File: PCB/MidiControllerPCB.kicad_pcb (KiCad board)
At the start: 2 copper layers, 202.8 x 137.6 mm, 62 parts, among them J1 OLED_Display, J2 fan_header, J24 TRS_Midi_1, J25 TRS_Midi_2, J3 TRS_Midi_3, J35 Raspberry_Pi_2_3, J4 TRS_Midi_4, J41 PIC_debug, J7 DIN_5, J8 DIN_5, SW1 SW_SPST, SW2 SW_SPST, SW3 SW_SPST, SW4 SW_SPST, SW5 SW_SPST, SW6 RGB_Rotary_Enc_PB, U10 PIC18F26K80_IML, U2 MCP23017_ML, U5 CD4050BCN

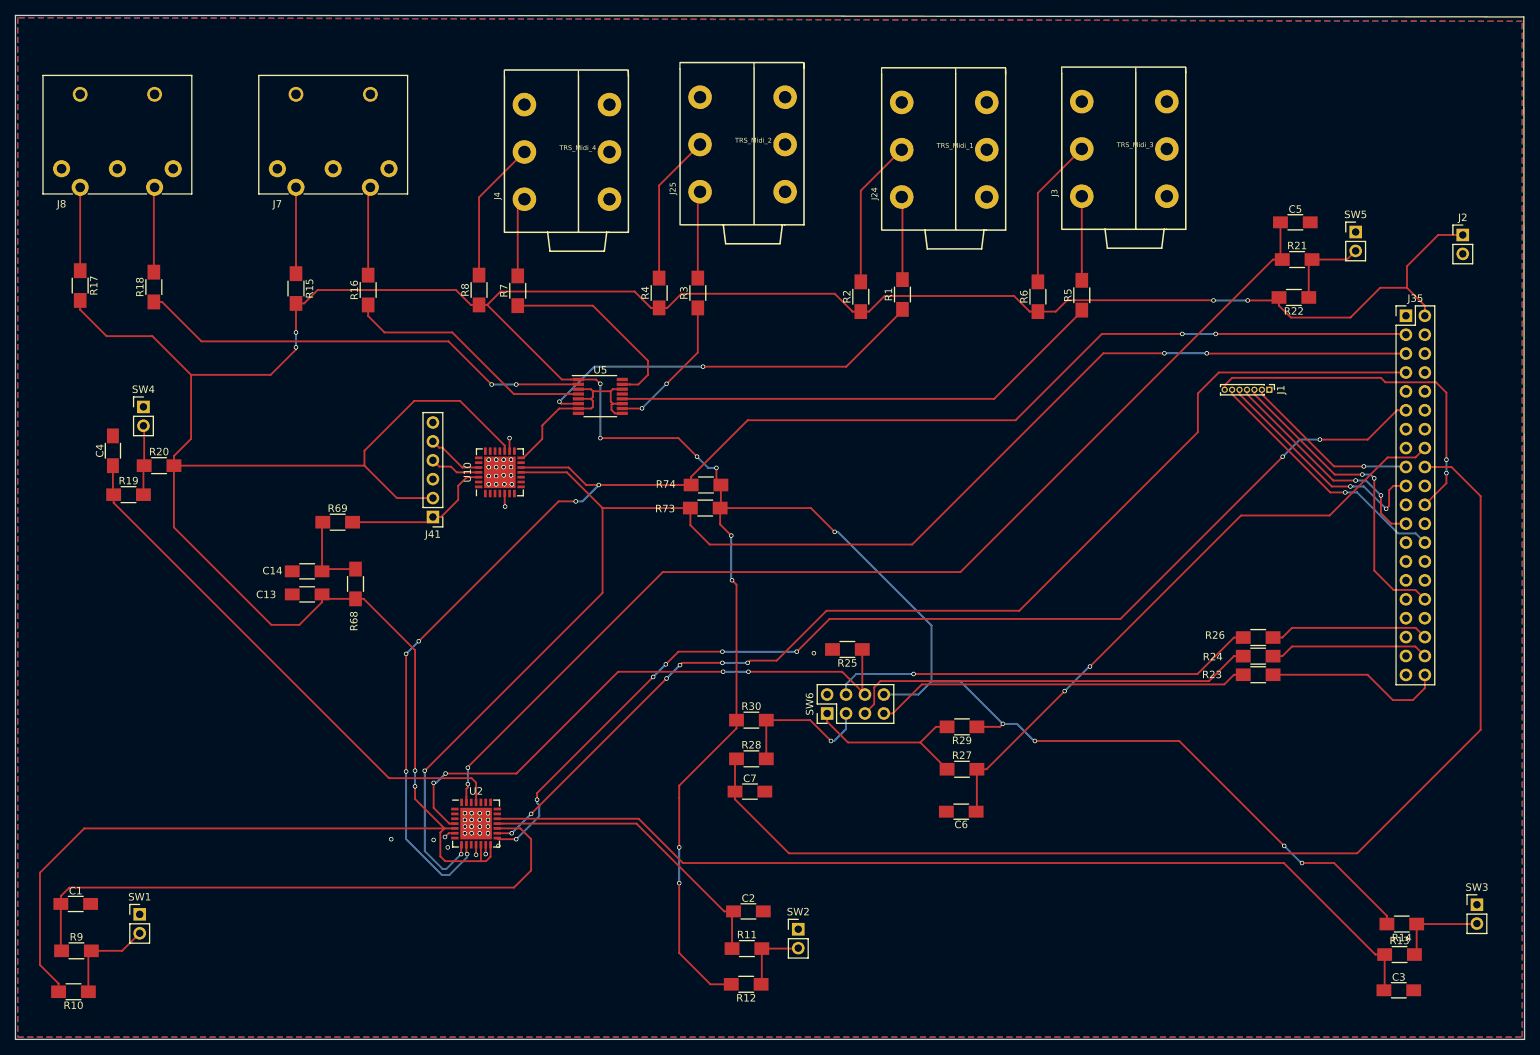
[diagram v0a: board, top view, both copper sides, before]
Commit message: modify pcb
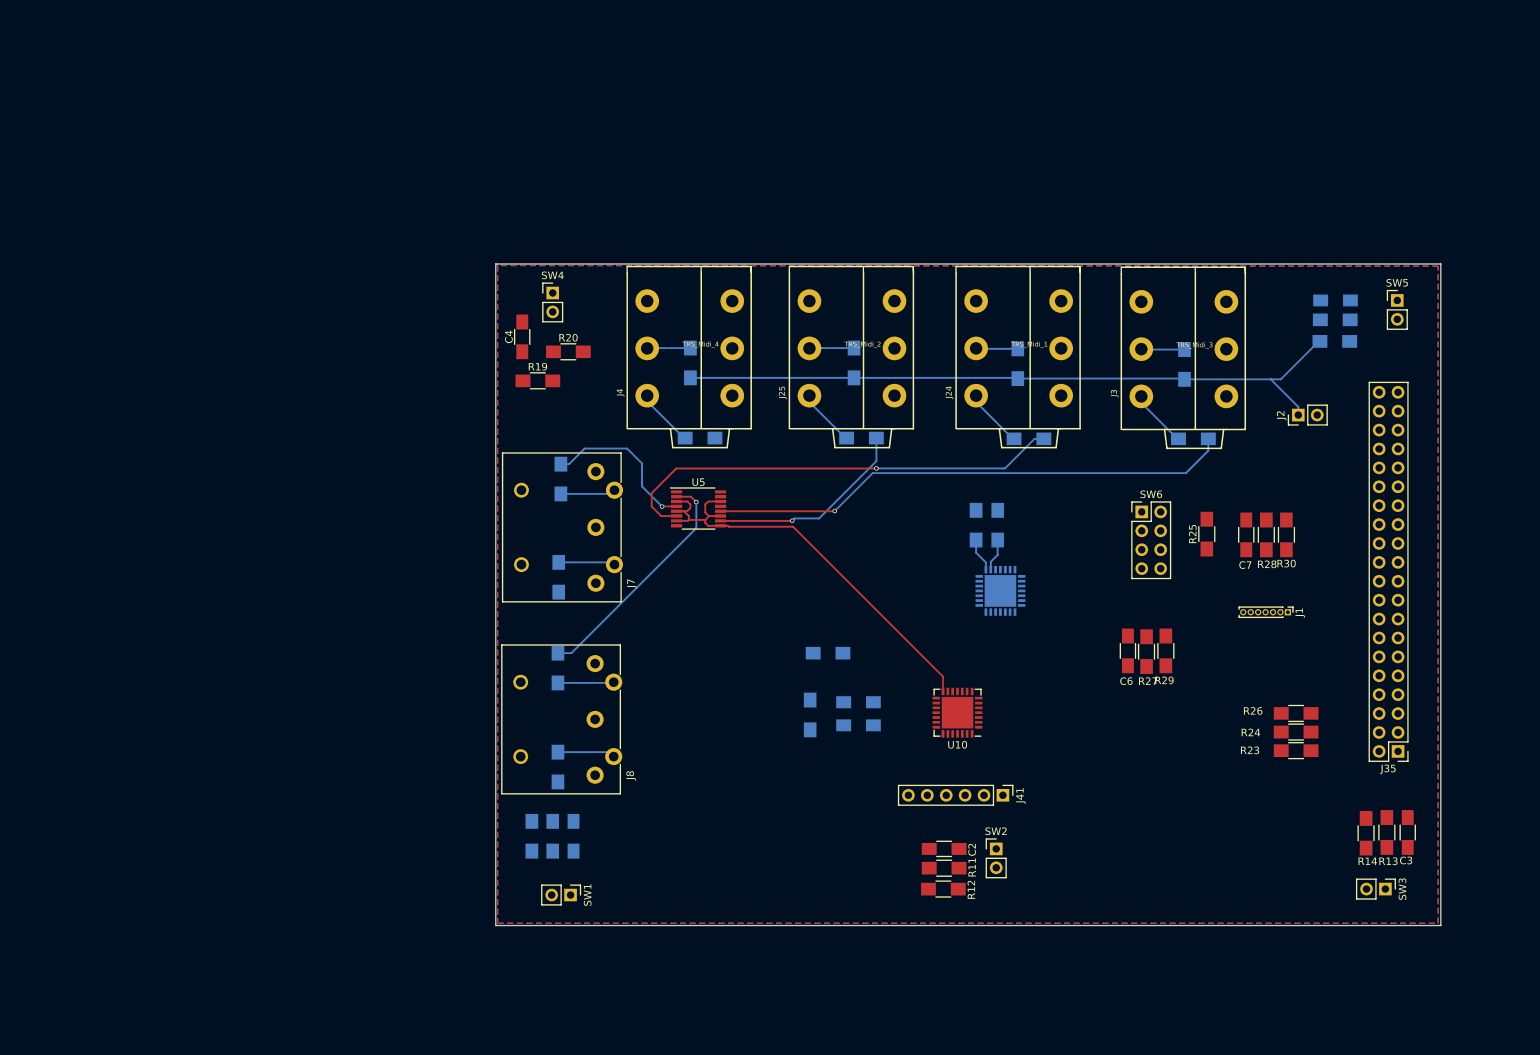
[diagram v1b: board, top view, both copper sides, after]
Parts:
- C1, C13, C14, C5, R1, R10, R15, R16, R17, R18, R2, R21, R22, R3, R4, R5, R6, R68, R69, R7, R73, R74, R8, R9, U2: moved to B.Cu
- moved J8 108.6 mm to (109.7, 123.9), turned to 90 degrees
- moved R17 91.1 mm to (104.7, 122.8)
- moved J41 85.2 mm to (164.5, 126.6), turned to 270 degrees
- moved U2 77.1 mm to (164.2, 99.1)
- moved C13 76.2 mm to (145.1, 117.2), turned to 180 degrees
- moved C14 76.2 mm to (145.1, 114.1), turned to 180 degrees
- moved R30 76.1 mm to (202.6, 91.6), turned to 270 degrees
- moved R28 75.5 mm to (199.9, 91.6), turned to 270 degrees
- moved C7 75.1 mm to (197.2, 91.6), turned to 270 degrees
- moved R18 74.6 mm to (104.7, 109.5), turned to 270 degrees
- moved J7 70.2 mm to (109.8, 98.1), turned to 90 degrees
- moved U10 69.5 mm to (158.4, 115.5), turned to 180 degrees
- moved R69 68.2 mm to (141.0, 107.5), turned to 180 degrees
- moved C1 67.5 mm to (106.8, 132.1), turned to 270 degrees
- moved R9 65.8 mm to (104.0, 132.1), turned to 270 degrees
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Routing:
- net VCC: track 713.8 -> 93.1 mm, vias 19 -> 0
- net Net-(J35-Pad3): track 202.1 -> 4.37 mm, vias 8 -> 0
- net Net-(J35-Pad5): track 198.9 -> 4.53 mm, vias 4 -> 0
- net RotEncB: track 156.1 -> 0.00 mm
- net Net-(J35-Pad7): track 150.8 -> 0.00 mm, vias 6 -> 0
- net Net-(J35-Pad11): track 148.3 -> 0.00 mm, vias 8 -> 0
- net FootSw5: track 147.6 -> 0.00 mm, vias 2 -> 0
- net FootSw3: track 131.7 -> 0.00 mm
- net RotEncA: track 83.8 -> 0.00 mm, vias 2 -> 0
- net FootSw1: track 81.4 -> 0.00 mm
- net RotEncPushBttn: track 78.7 -> 0.00 mm, vias 4 -> 0
- net FootSw4: track 72.0 -> 0.00 mm
- net Net-(R26-Pad1): track 57.4 -> 0.00 mm, vias 1 -> 0
- net Net-(R24-Pad1): track 55.4 -> 0.00 mm
- net Net-(R23-Pad1): track 50.5 -> 0.00 mm
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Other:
- board size 202.8 x 137.6 mm -> 127 x 88.9 mm
